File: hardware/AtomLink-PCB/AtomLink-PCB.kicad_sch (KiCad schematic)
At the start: 24 parts, among them J1 Conn_01x03, J2 Atom1, J3 Atom2, J4 PF cable, Q1 AS2309, Q2 MUN5235, Q3 AS2309, Q4 MUN5235, U1 LMZM23600V5

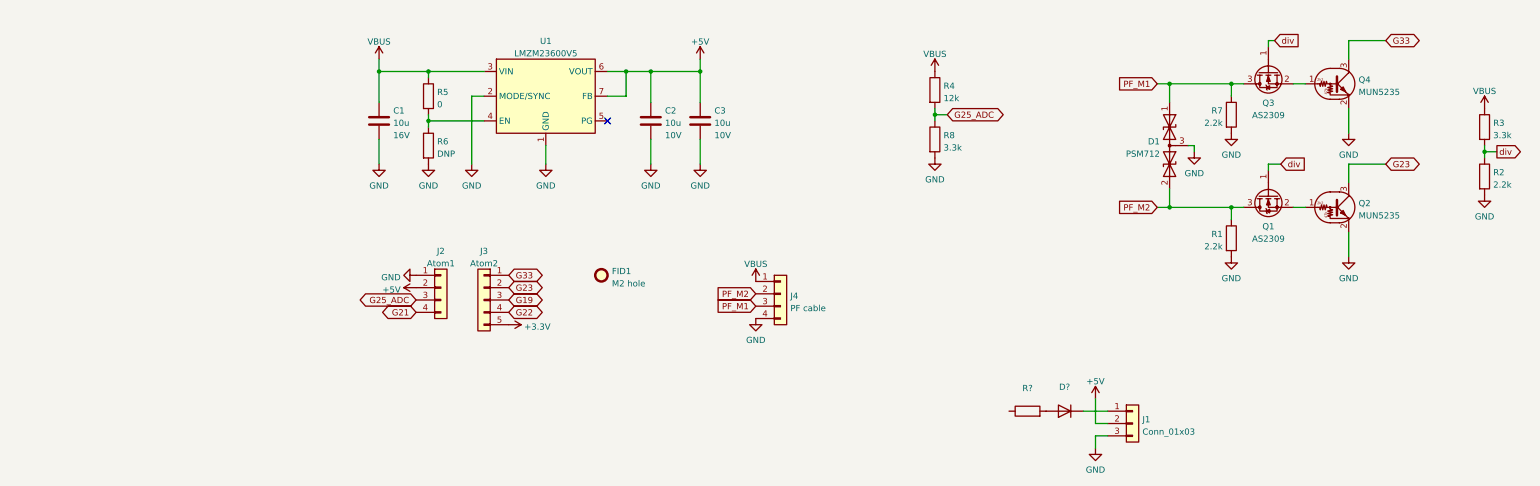
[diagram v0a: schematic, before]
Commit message: Schematic & layout changes
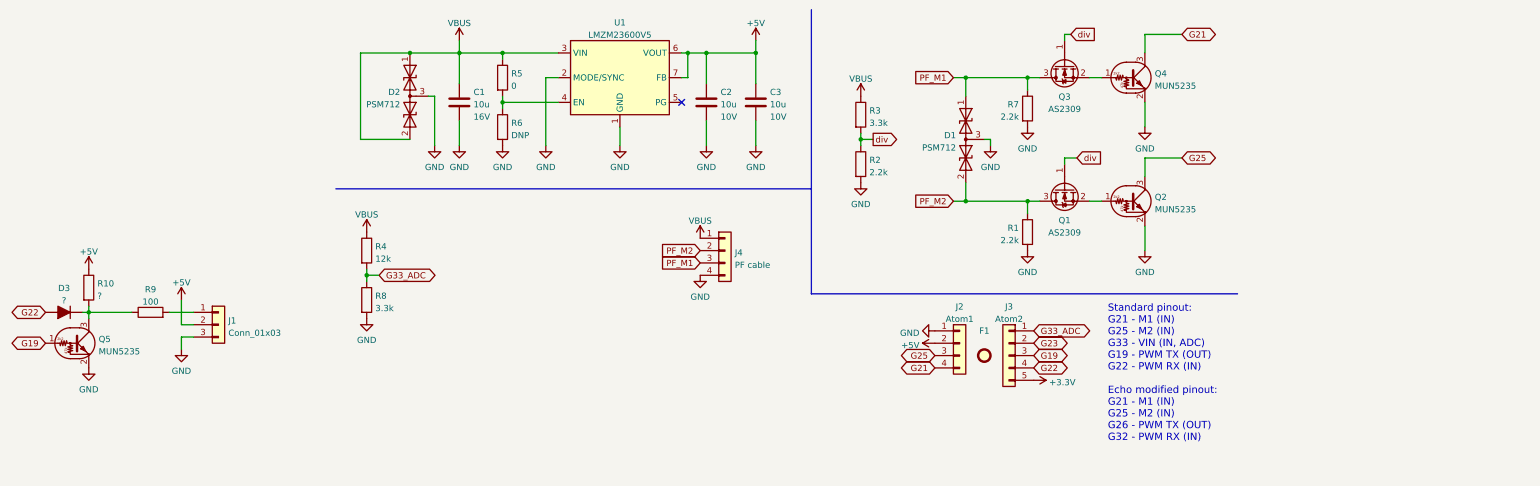
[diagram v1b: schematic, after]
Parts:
- removed D?: (no value), symbol Device:D
- added D2: PSM712, Package_TO_SOT_SMD:SOT-23, symbol Diode:SM712_SOT23
- added D3: ?, symbol Device:D_Filled
- added Q5: MUN5235, Package_TO_SOT_SMD:SOT-323_SC-70, symbol Transistor_BJT:DTC123J
- added R10: ?, Resistor_SMD:R_0402_1005Metric, symbol Device:R
- F1: renamed from FID1; value M2 hole -> (none)
- R9: renamed from R?; value (none) -> 100
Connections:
- net +5V: now also R10.1
- net G19: now also Q5.1 (B)
- net G21: now also Q4.3 (C)
- net G22: now also D3.2 (A)
- net G23: no longer Q2.3 (C)
- net GND: now also D2.3 (common), Q5.2 (E)
- net VBUS: now also D2.1 (A1), D2.2 (A2)
- net at J1.1 (Pin_1): now also R9.2
- net at R9.1: now also D3.1 (K), Q5.3 (C), R10.2
- net G25_ADC renamed G33_ADC
- net G33_ADC: now also J3.1 (Pin_1); no longer J2.3 (Pin_3)
- removed net G33: J3.1 (Pin_1), Q4.3 (C)
- new net G25: J2.3 (Pin_3), Q2.3 (C)
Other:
- note added: "Standard pinout: G21 - M1 (IN) G25 - M2 (IN) G33 - VIN (IN, ADC) G19 - PWM TX (OUT) G22 - PWM RX (IN) Echo modified pinout: G21 - M1 (IN) G25 - M2 (IN) G26 - PWM TX (OUT) G32 - PWM RX (IN)"
- moved on the sheet: C1, C2, C3, D1, F1, J1, J2, J3, J4, Q1, Q2, Q3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
